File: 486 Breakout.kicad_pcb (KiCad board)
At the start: 4 copper layers, 100 x 100 mm, 50 parts, among them J1 PWR, J10 Conn_02x03_Counter_Clockwise, J11 Byte Enabled, J12 FPU, J13 Input, J14 Bus Size, J15 Bus Arbitration, J2 Conn_02x04_Counter_Clockwise, J3 Not Connected, J4 Address Bus, J5 Data Bus, J6 Conn_02x03_Counter_Clockwise, J7 Control Bus, J8 Cache, J9 Parity, U1 80486DX, U2 7400, U3 7400

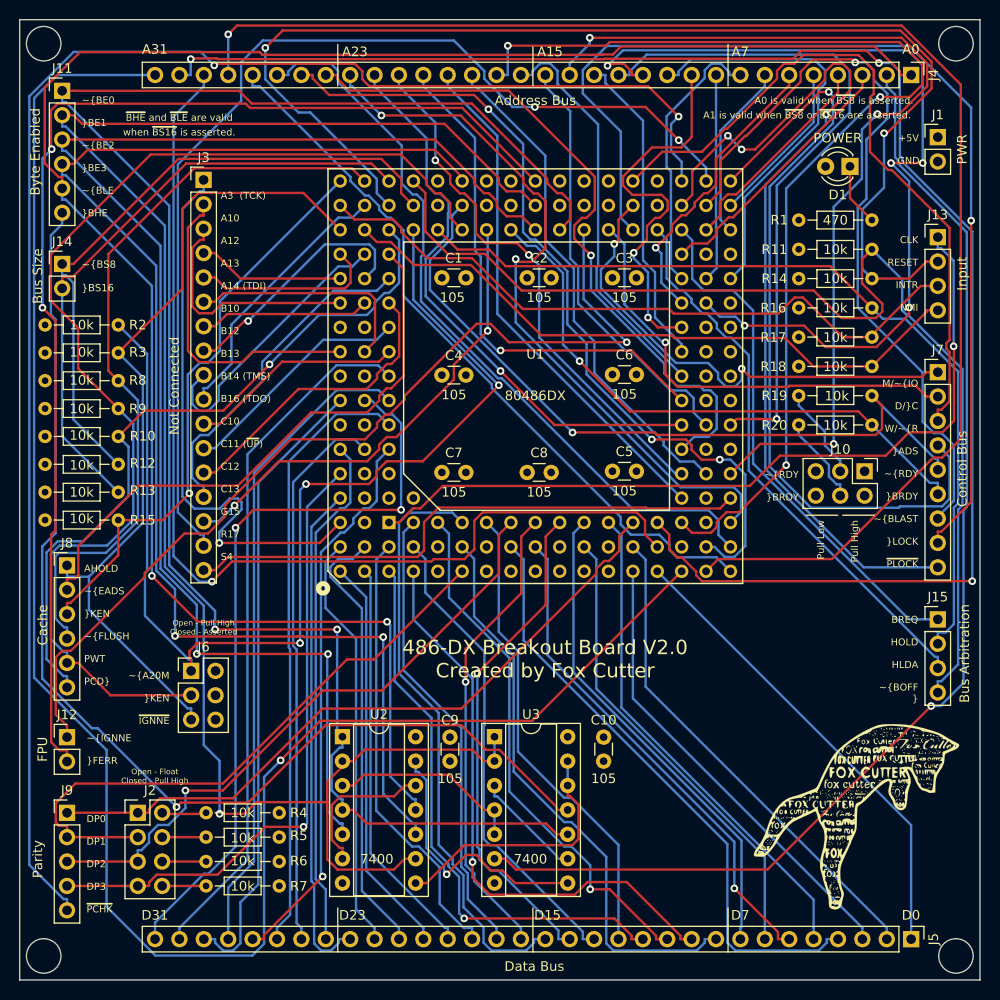
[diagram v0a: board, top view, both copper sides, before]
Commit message: * Update to Kicad 6
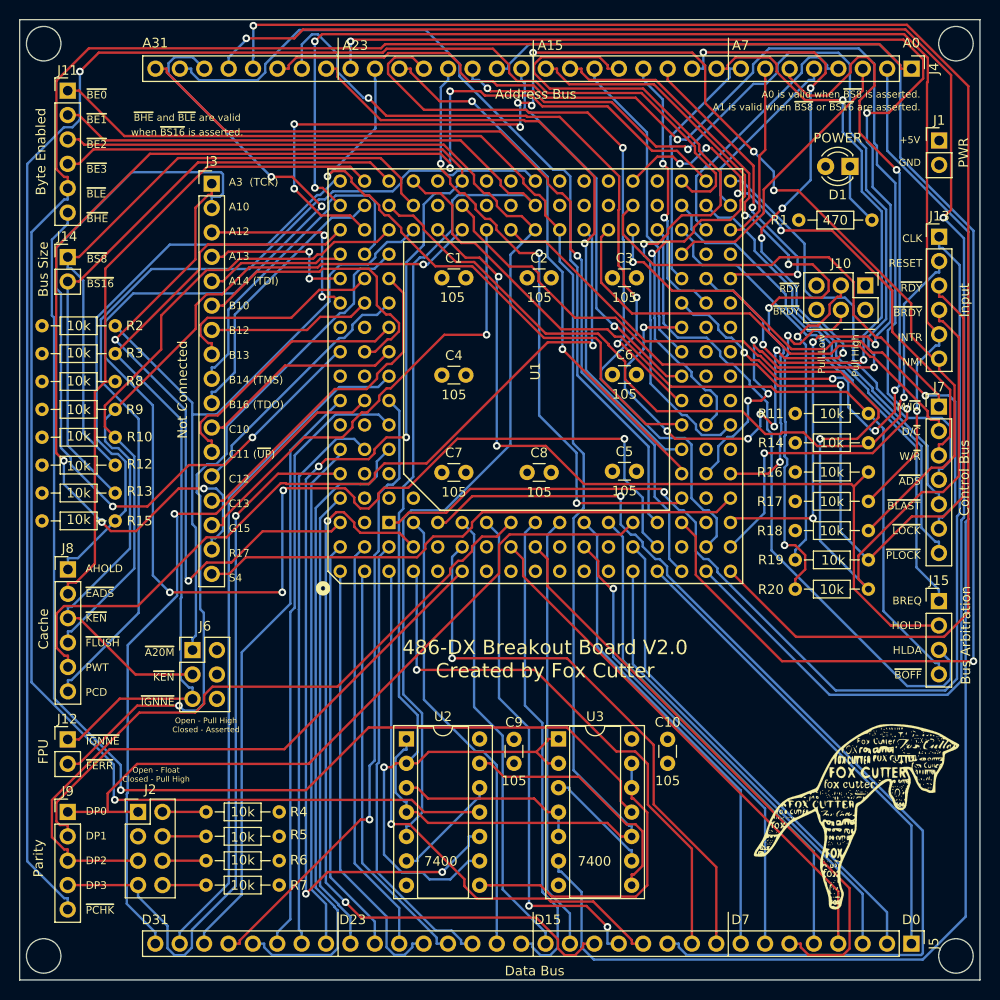
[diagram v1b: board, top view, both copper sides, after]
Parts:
- J13: footprint Connector_PinHeader_2.54mm:PinHeader_1x04_P2.54mm_Vertical -> Connector_PinHeader_2.54mm:PinHeader_1x06_P2.54mm_Vertical
- J7: footprint Connector_PinHeader_2.54mm:PinHeader_1x09_P2.54mm_Vertical -> Connector_PinHeader_2.54mm:PinHeader_1x07_P2.54mm_Vertical
- U1: footprint 486:PGA169 -> 486 Breakout:PGA169
- moved J10 19.4 mm to (158.1, 77.7)
- moved R11 17.1 mm to (158.4, 91.0)
- moved R14 17.1 mm to (158.4, 94.1)
- moved R16 17.1 mm to (158.4, 97.1)
- moved R17 17.1 mm to (158.4, 100.2)
- moved R18 17.1 mm to (158.4, 103.2)
- moved R19 17.1 mm to (158.4, 106.3)
- moved R20 17.1 mm to (158.4, 109.3)
- moved U2 6.67 mm to (110.3, 124.9)
- moved U3 6.67 mm to (126.1, 124.9)
- moved C10 6.67 mm to (137.5, 124.9)
- moved C9 6.67 mm to (121.5, 124.9)
- moved J7 3.59 mm to (165.7, 90.3)
- moved J6 2.17 mm to (88.0, 115.7)
- moved J15 1.90 mm to (165.7, 110.5)
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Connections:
- J12 pad 1: PWT -> IGNNE#
- J12 pad 2: PCD -> FERR#
- J13 pad 3: INTR -> RDY#
- J13 pad 4: NMI -> BRDY#
- J7 pad 5: RDY# -> BLAST#
- J7 pad 6: BRDY# -> LOCK#
- J7 pad 7: BLAST# -> PLOCK#
- J8 pad 1: IGNNE# -> AHOLD
- J8 pad 2: FERR# -> EADS#
- J8 pad 3: AHOLD -> KEN#
- J8 pad 4: EADS# -> FLUSH#
- J8 pad 5: KEN# -> PWT
- J8 pad 6: FLUSH# -> PCD
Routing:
- net A31: track 189.7 -> 92.8 mm
- net A27: track 77.3 -> 165.1 mm, vias 0 -> 1
- net A30: track 170.7 -> 90.9 mm, vias 3 -> 0
- net NMI: track 68.1 -> 133.4 mm, vias 0 -> 8
- net A11: track 93.1 -> 28.3 mm, vias 5 -> 2
- net A18: track 52.8 -> 115.2 mm, vias 0 -> 6
- net INTR: track 71.9 -> 133.8 mm, vias 0 -> 3
- net A26: track 79.1 -> 139.1 mm, vias 0 -> 3
- net A9: track 40.0 -> 99.8 mm, vias 2 -> 11
- net A23: track 76.3 -> 132.7 mm, vias 2 -> 5
- net D10: track 55.6 -> 108.7 mm
- net LOCK#: track 109.9 -> 57.8 mm, vias 1 -> 2
- net NC1: track 33.0 -> 85.0 mm, vias 0 -> 2
- net A5: track 31.2 -> 82.3 mm, vias 1 -> 5
- net A29: track 110.0 -> 160.9 mm, vias 1 -> 6
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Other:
- net class +5V removed
- net class Default removed
- net class GND removed
- board text added: "A0 is valid when ~{BS8} is asserted."
- board text added: "A1 is valid when ~{BS8} or ~{BS16} are asserted."
- board text added: "A3 (TCK) A10 A12 A13 A14 (TDI) B10 B12 B13 B14 (TMS) B16 (TDO) C10 C11 (~{UP}) C12 C13 G15 R17 S4"
- board text added: "AHOLD ~{EADS} ~{KEN} ~{FLUSH} PWT PCD"
- board text added: "BREQ HOLD HLDA ~{BOFF}"
- board text added: "CLK RESET ~{RDY} ~{BRDY} INTR NMI"
- board text added: "DP0 DP1 DP2 DP3 ~{PCHK}"
- board text added: "M/~{IO} D/~{C} W/~{R} ~{ADS} ~{BLAST} ~{LOCK} ~{PLOCK}"
- board text added: "when ~{BS16} is asserted."
- board text added: "~{A20M} ~{KEN} ~{IGNNE}"
- board text added: "~{BE0} ~{BE1} ~{BE2} ~{BE3} ~{BLE} ~{BHE}"
- board text added: "~{BHE} and ~{BLE} are valid"
- board text added: "~{BS8} ~{BS16}"
- board text added: "~{IGNNE} ~{FERR}"
- board text added: "~{RDY} ~{BRDY}"
- board text removed: "A0 is valid when ~BS8~ is asserted."
- board text removed: "A1 is valid when ~BS8~ or ~BS16~ are asserted."
- board text removed: "A3 (TCK) A10 A12 A13 A14 (TDI) B10 B12 B13 B14 (TMS) B16 (TDO) C10 C11 (~UP~) C12 C13 G15 R17 S4"
- board text removed: "AHOLD ~EADS ~KEN ~FLUSH PWT PCD"
- board text removed: "BREQ HOLD HLDA ~BOFF"
- board text removed: "CLK RESET INTR NMI"
- board text removed: "DP0 DP1 DP2 DP3 ~PCHK"
- board text removed: "M/~IO D/~C W/~R ~ADS ~RDY ~BRDY ~BLAST ~LOCK ~PLOCK"
- board text removed: "when ~BS16~ is asserted."
- board text removed: "~A20M ~KEN ~IGNNE"
- board text removed: "~BE0 ~BE1 ~BE2 ~BE3 ~BLE ~BHE"
- board text removed: "~BHE~ and ~BLE~ are valid"
- board text removed: "~BS8 ~BS16"
- board text removed: "~IGNNE ~FERR"
- board text removed: "~RDY ~BRDY"
